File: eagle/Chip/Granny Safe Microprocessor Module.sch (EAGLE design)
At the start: 45 parts, among them IC1 MCP604SL, J1 3x4 Keypad, J3 SCREW-4, J6 FEMALE 2x3, Q1 TRANS_NPN-MMBTA42, Q2 TRANS_NPN-MMBTA42, Q3 TRANS_NPN-MMBTA42, U1 328P, Y1 16MHz

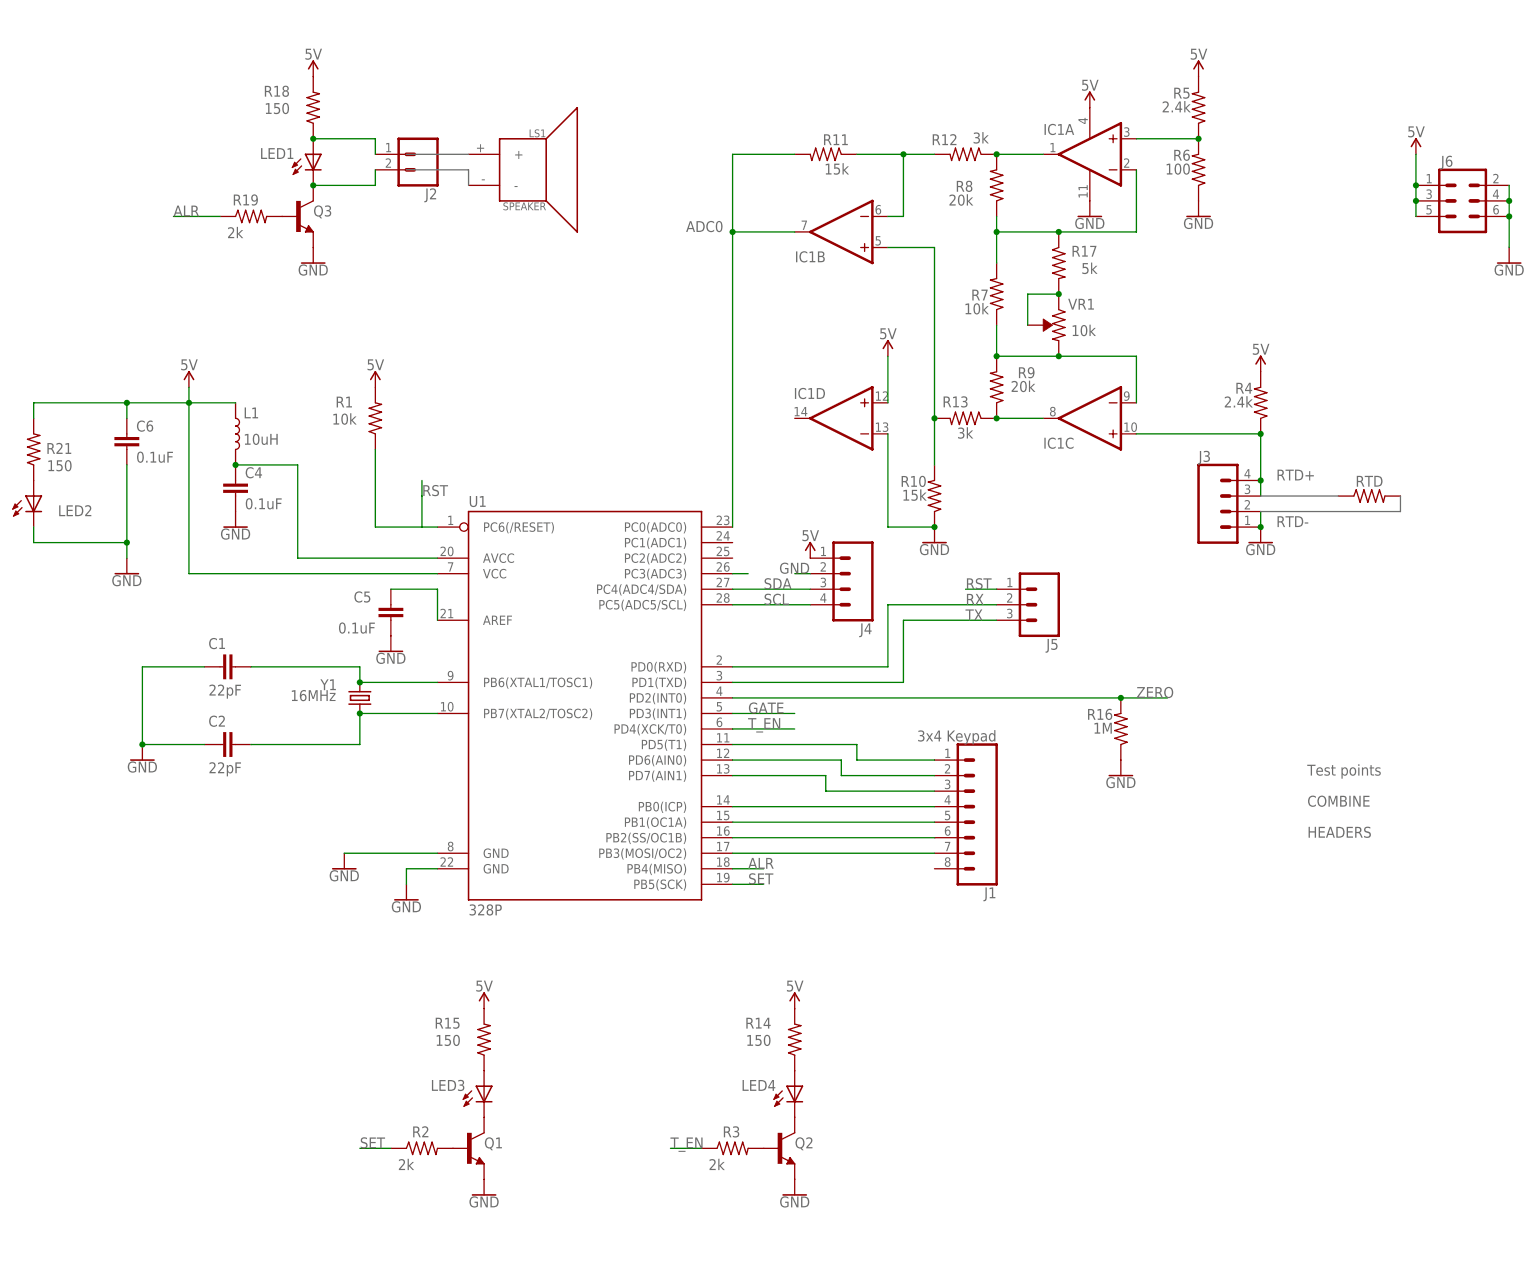
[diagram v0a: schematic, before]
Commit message: Put both schematics together
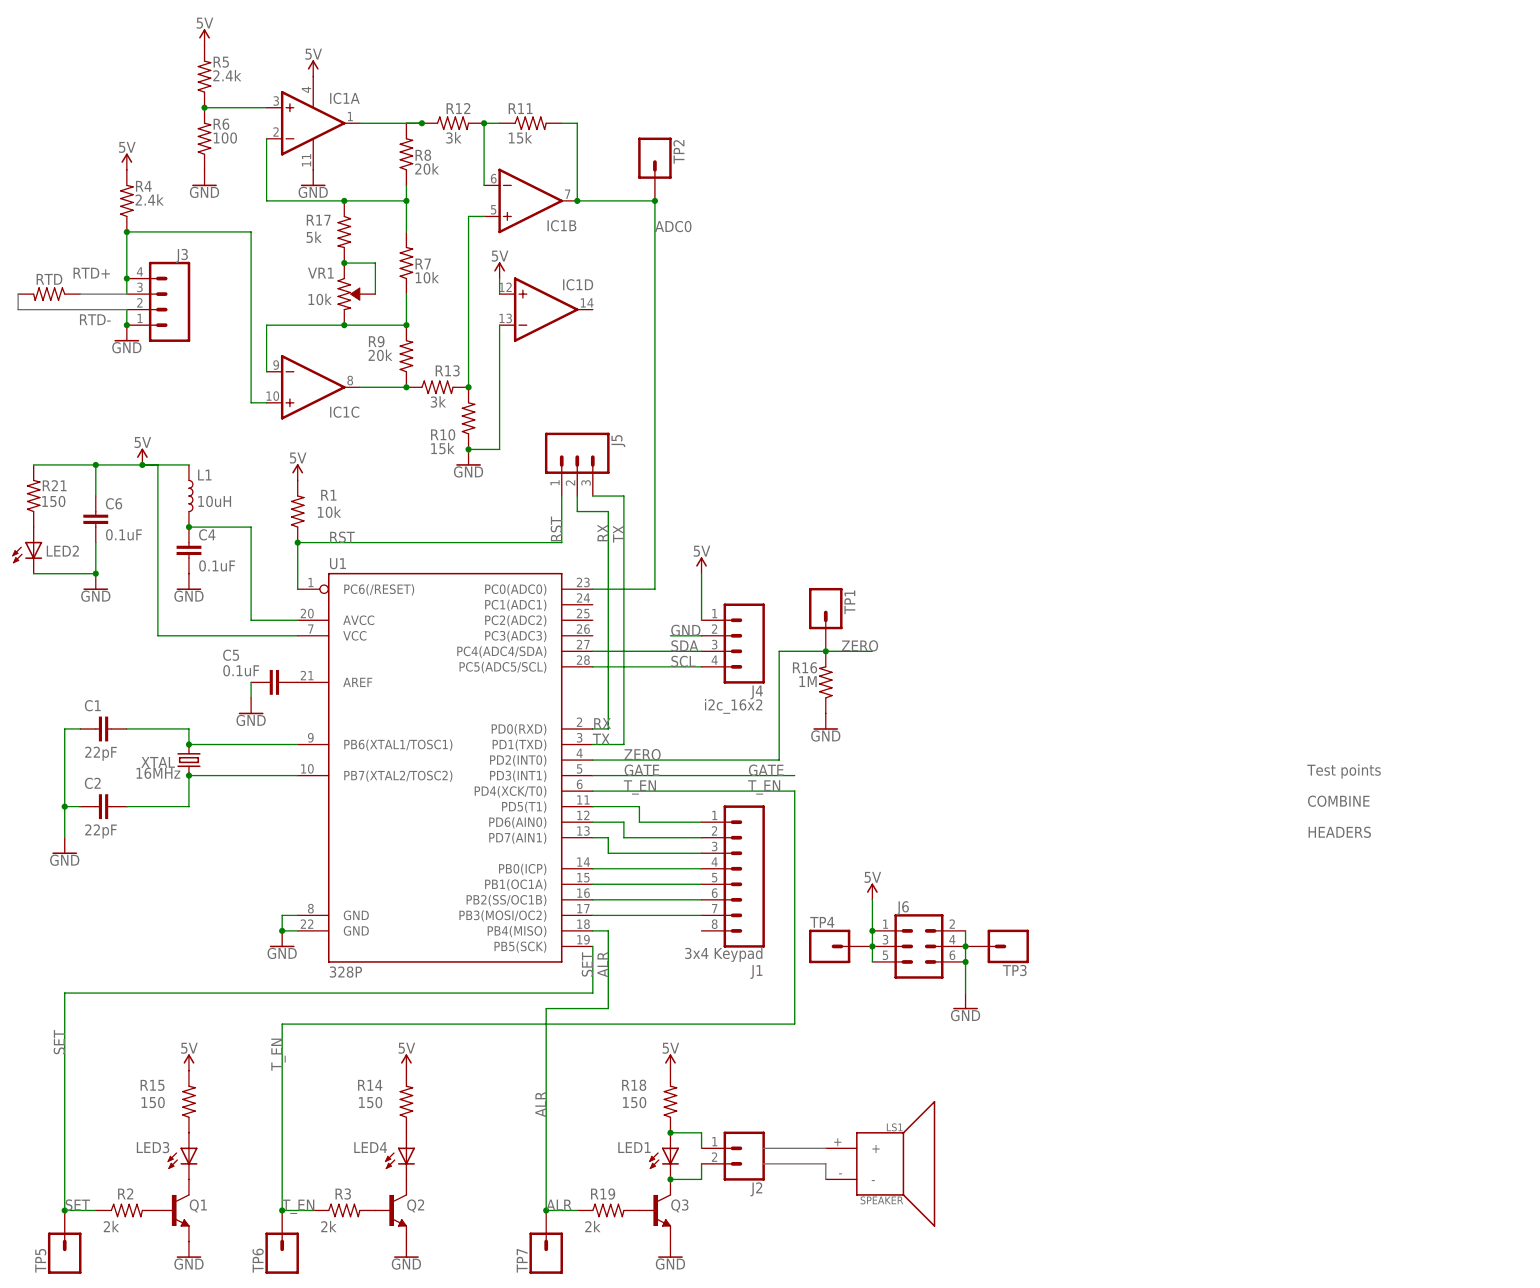
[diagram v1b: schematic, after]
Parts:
- removed Y1: 16MHz, SparkFun-Clocks:CRYSTAL-16MHZPTH-HC49US
- added TP1, TP2, TP3, TP4, TP5, TP6, TP7: (no value), SparkFun-Connectors:CONN_01
- added XTAL: 16MHz, SparkFun-Clocks:CRYSTAL-16MHZPTH-HC49US
- J4: value (none) -> i2c_16x2
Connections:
- removed net N$50: U1.PC3(ADC3)
- net 5V: now also TP4.1
- net ADC0: now also TP2.1
- net ALR: now also TP7.1
- net GND: now also TP3.1
- net N$1: now also XTAL.2; no longer Y1.2
- net N$2: now also XTAL.1; no longer Y1.1
- net SET: now also TP5.1
- net T_EN: now also TP6.1
- net ZERO: now also TP1.1
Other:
- note removed: "ADC0"
- moved on the sheet: C1, C2, C4, C5, C6, IC1A, IC1B, IC1C, IC1D, J1, J2, J3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
